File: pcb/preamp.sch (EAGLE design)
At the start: 50 parts, among them U1 LT1097CN8PBF, U2 LT1097CN8PBF, U3 LT1079CNPBF, U4 LT1079CNPBF

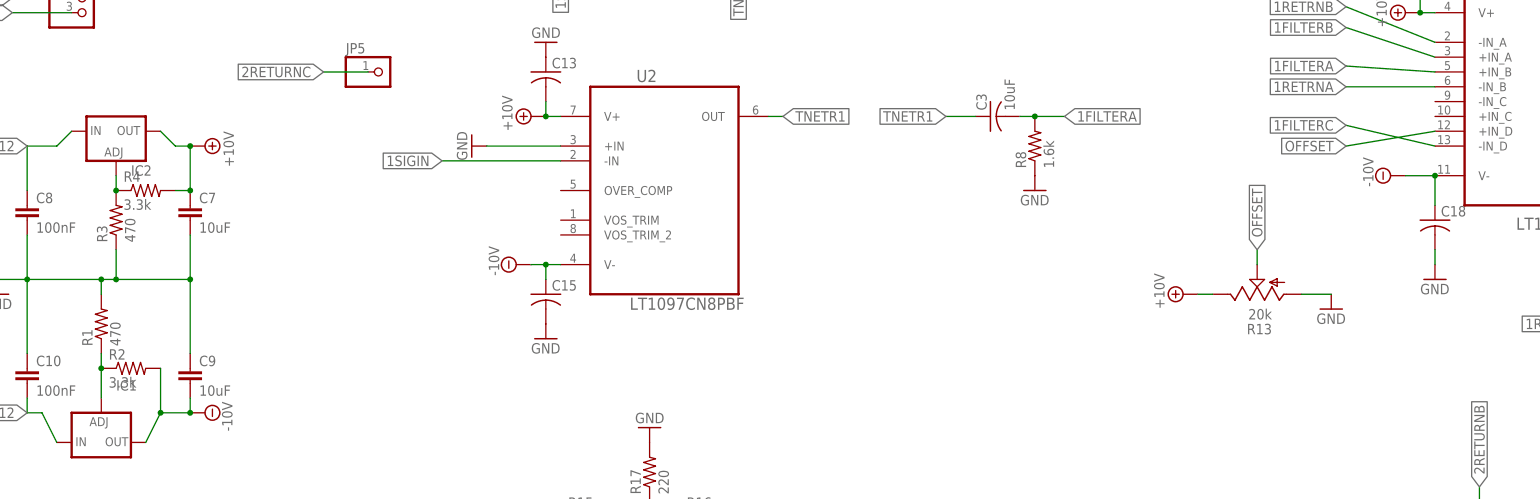
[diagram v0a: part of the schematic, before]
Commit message: some circuit modifications, updates
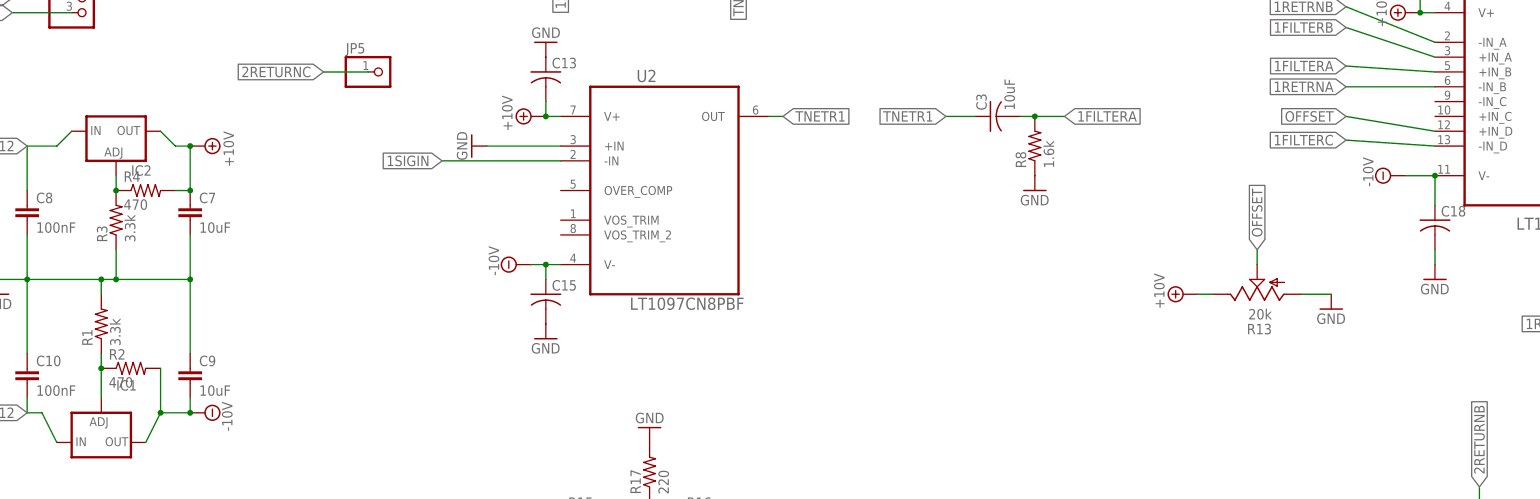
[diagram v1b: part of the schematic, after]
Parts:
- R1, R3: value 470 -> 3.3k
- R2, R4: value 3.3k -> 470
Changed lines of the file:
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@@
 <?xml version="1.0" encoding="utf-8"?>
 <!DOCTYPE eagle SYSTEM "eagle.dtd">
-<eagle version="6.6.0">
+<eagle version="7.3.0">
 <drawing>
 <settings>
@@
 <part name="SUPPLY6" library="supply2" deviceset="+10V" device=""/>
 <part name="GND1" library="supply1" deviceset="GND" device=""/>
-<part name="R1" library="resistor" deviceset="R-US_" device="0204/5" value="470"/>
-<part name="R2" library="resistor" deviceset="R-US_" device="0204/5" value="3.3k"/>
-<part name="R3" library="resistor" deviceset="R-US_" device="0204/5" value="470"/>
-<part name="R4" library="resistor" deviceset="R-US_" device="0204/5" value="3.3k"/>
+<part name="R1" library="resistor" deviceset="R-US_" device="0204/5" value="3.3k"/>
+<part name="R2" library="resistor" deviceset="R-US_" device="0204/5" value="470"/>
+<part name="R3" library="resistor" deviceset="R-US_" device="0204/5" value="3.3k"/>
+<part name="R4" library="resistor" deviceset="R-US_" device="0204/5" value="470"/>
 <part name="R8" library="resistor" deviceset="R-US_" device="0204/5" value="1.6k"/>
 <part name="R9" library="resistor" deviceset="R-US_" device="0204/5" value="16.2k"/>
@@
 <net name="1FILTERC" class="0">
 <segment>
-<label x="154.94" y="87.376" size="1.778" layer="95" rot="R180" xref="yes"/>
+<label x="154.94" y="84.836" size="1.778" layer="95" rot="R180" xref="yes"/>
 <pinref part="U3" gate="A" pin="-IN_D"/>
-<wire x1="170.18" y1="83.82" x2="154.94" y2="87.376" width="0.1524" layer="91"/>
+<wire x1="170.18" y1="83.82" x2="154.94" y2="84.836" width="0.1524" layer="91"/>
 </segment>
 <segment>
@@
 <net name="OFFSET" class="0">
 <segment>
-<label x="154.94" y="83.82" size="1.778" layer="95" rot="R180" xref="yes"/>
+<label x="154.94" y="88.9" size="1.778" layer="95" rot="R180" xref="yes"/>
 <pinref part="U3" gate="A" pin="+IN_D"/>
-<wire x1="170.18" y1="86.36" x2="154.94" y2="83.82" width="0.1524" layer="91"/>
-</segment>
-<segment>
+<wire x1="170.18" y1="86.36" x2="154.94" y2="88.9" width="0.1524" layer="91"/>
+</segment>
+<segment>
